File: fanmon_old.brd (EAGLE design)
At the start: 77.1 x 55.9 mm, 33 parts, among them IC1 PIC18F1220P, IC2 5vdc reg, K1 G6D-1A-ASI5VDC, X1 22-23-2021, X2 22-23-2021, X3 22-23-2021, X4 22-23-2021, X5 22-23-2041

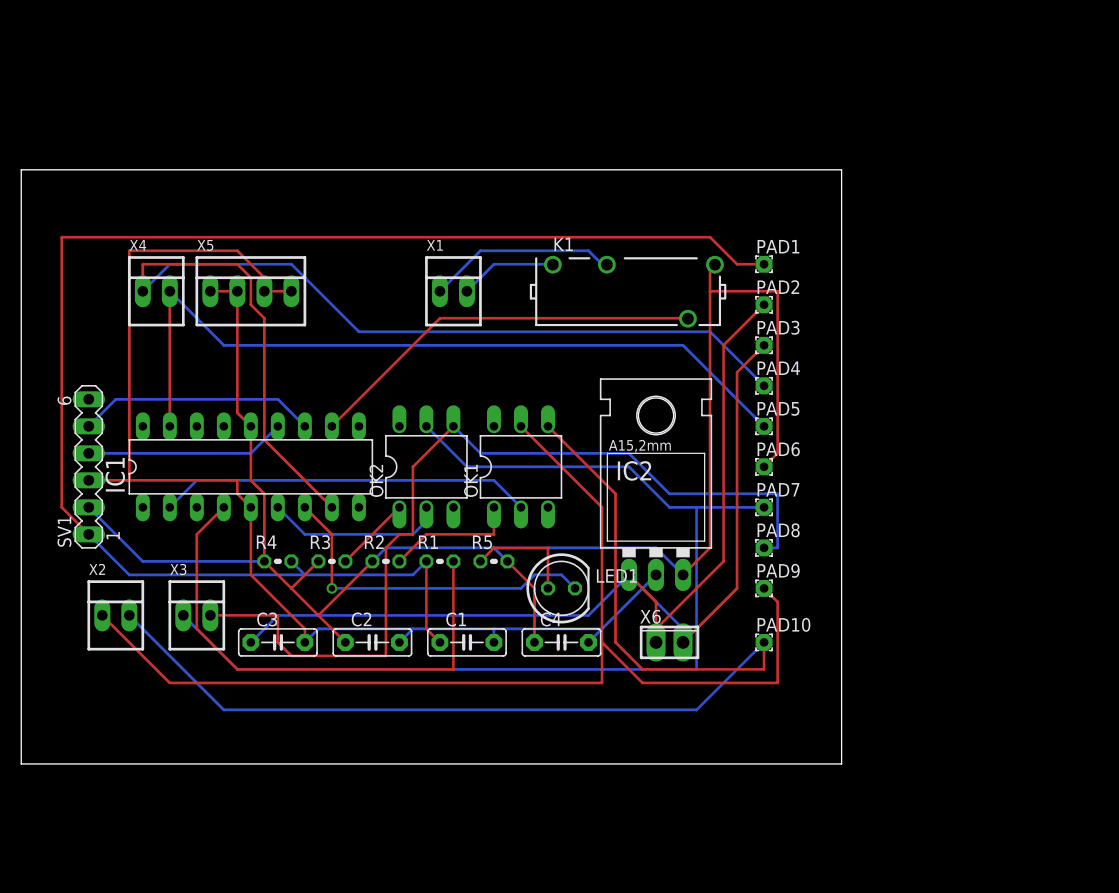
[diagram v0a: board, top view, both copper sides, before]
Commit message: updates
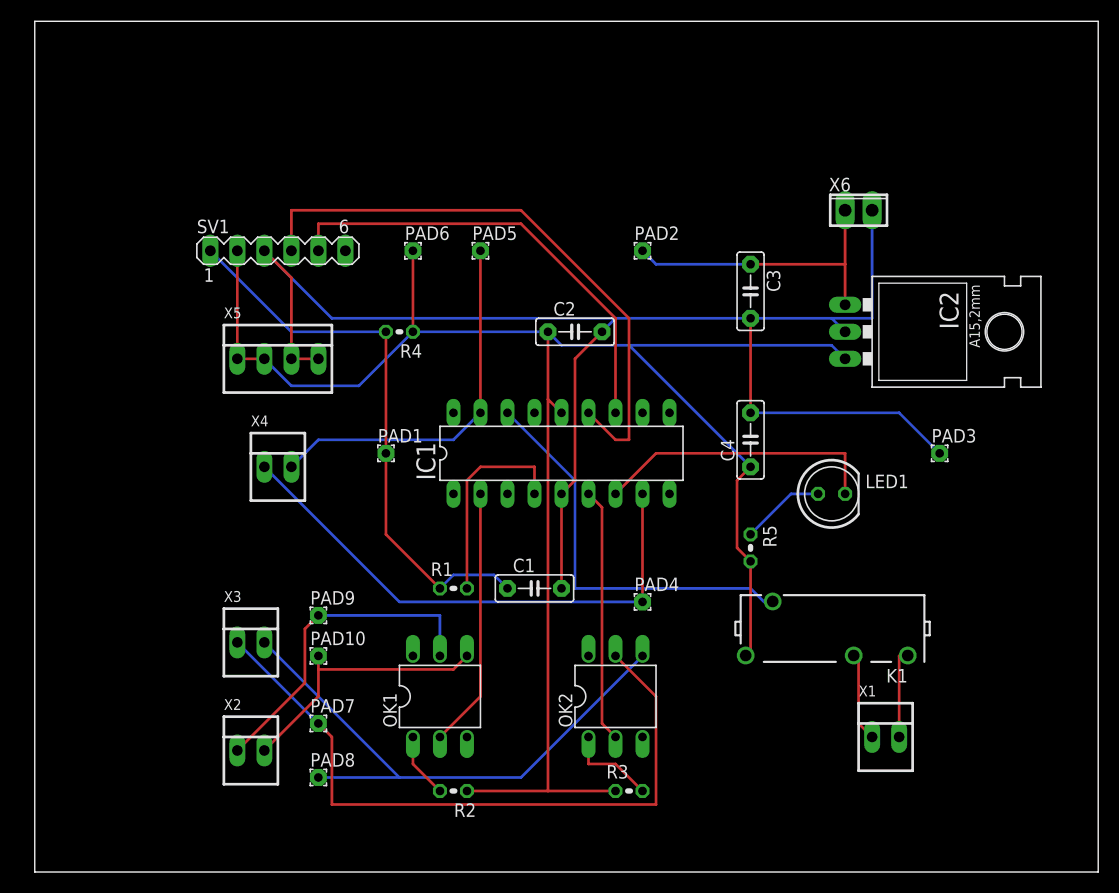
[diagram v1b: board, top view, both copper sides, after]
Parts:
- moved X1 58.4 mm to (80.0, 12.7)
- moved C3 55.4 mm to (67.3, 54.6), turned to 270 degrees
- moved PAD8 47.1 mm to (26.7, 8.89)
- moved PAD7 46.6 mm to (26.7, 14.0)
- moved X6 44.4 mm to (77.5, 62.2)
- moved PAD9 42.0 mm to (26.7, 24.1)
- moved PAD10 41.9 mm to (26.7, 20.3)
- moved PAD1 39.8 mm to (33.0, 39.4)
- moved PAD6 38.8 mm to (35.6, 58.4)
- moved K1 37.0 mm to (74.9, 22.9), turned to 180 degrees
- moved R3 35.3 mm to (55.9, 7.62)
- moved C2 34.9 mm to (50.8, 50.8)
- moved PAD5 31.4 mm to (41.9, 58.4)
- moved IC1 29.2 mm to (49.5, 39.4)
- moved IC2 28.8 mm to (80.0, 50.8), turned to 270 degrees
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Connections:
- net N$16: now also IC1.16; no longer IC1.11
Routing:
- net N$4: track 139.9 -> 53.3 mm
- net N$13: track 106.5 -> 25.5 mm
- net N$12: track 104.4 -> 31.1 mm
- net N$6: track 80.3 -> 28.5 mm
- net N$5: track 102.2 -> 51.0 mm
- net N$7: track 73.8 -> 35.1 mm
- net N$20: track 18.8 -> 56.1 mm
- net N$10: track 100.5 -> 65.0 mm
- net N$11: track 84.0 -> 53.2 mm
- net N$1: track 48.4 -> 19.6 mm
- net N$21: track 22.4 -> 43.1 mm
- net N$8: track 35.1 -> 24.4 mm
- net N$18: track 17.8 -> 8.61 mm
- net VDD: track 164.5 -> 173.5 mm
- net VSS: track 149.3 -> 141.2 mm
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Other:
- board size 77.1 x 55.9 mm -> 100 x 80 mm
